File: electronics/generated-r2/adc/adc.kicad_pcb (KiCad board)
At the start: 2 copper layers, 80 x 50 mm, 22 parts, among them J1 SPI_POWER, J2 8X_HALL_3V3_GND_SIGNAL, U1 MCP3208-BI/SL, U2 SN74LVC1G125DBVR_IOFF

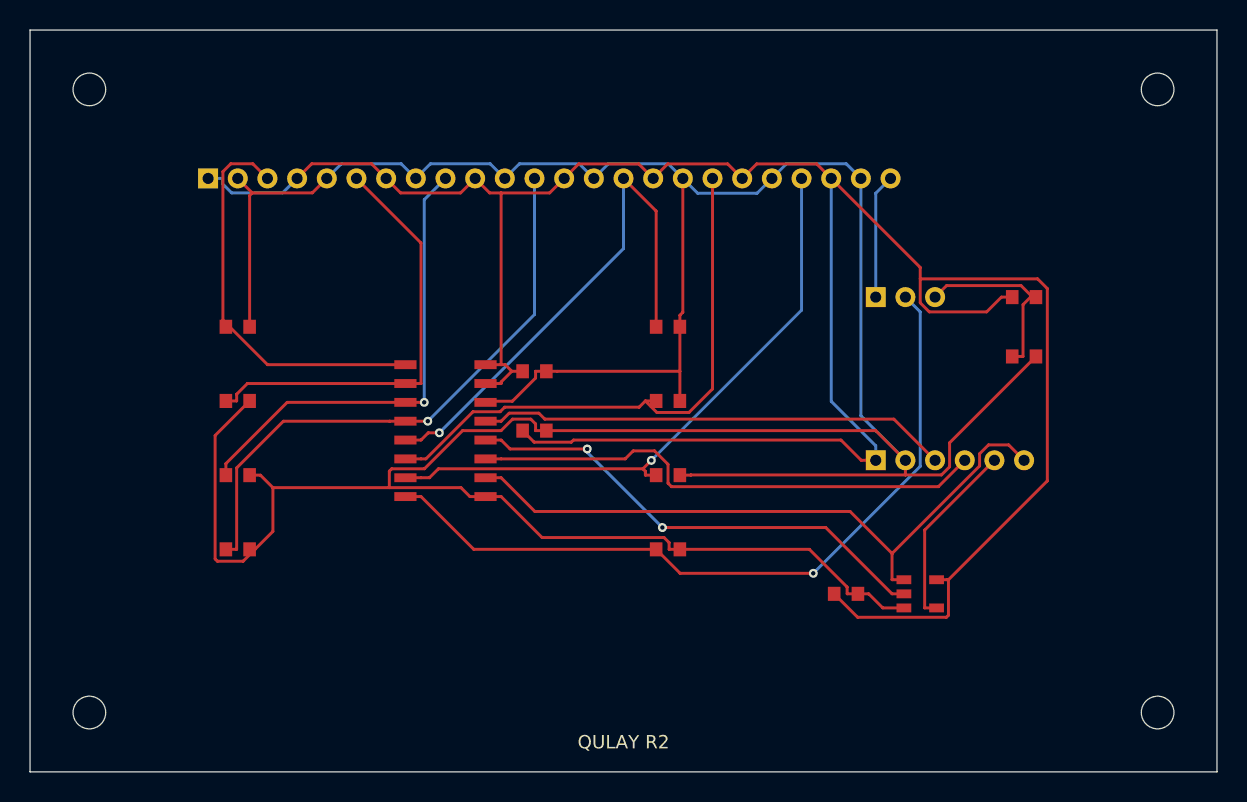
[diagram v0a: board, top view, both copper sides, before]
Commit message: build(r2): publish final routed electronics and checks [skip ci]
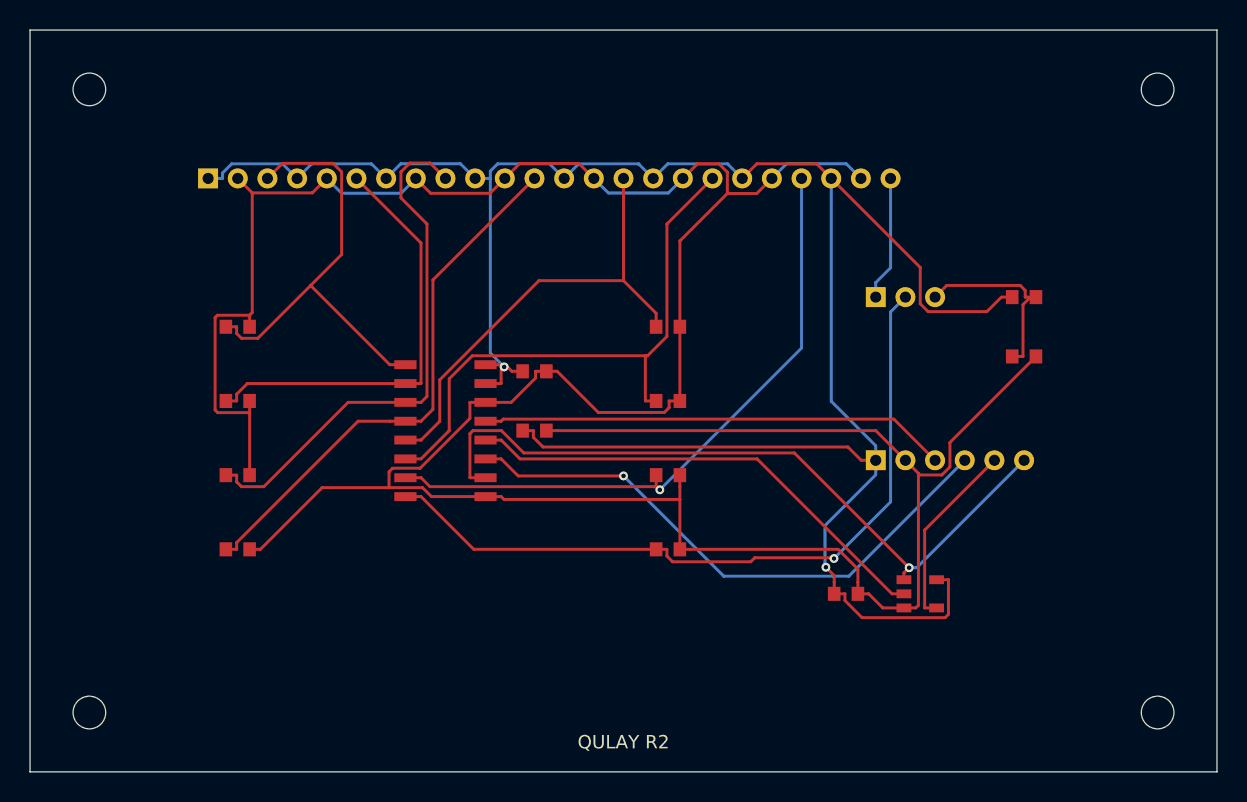
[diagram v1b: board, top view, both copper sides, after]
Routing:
- net GND: track 242.4 -> 218.1 mm
- net SENS_3V3: track 169.9 -> 151.6 mm, vias 0 -> 2
- net A2: track 31.5 -> 36.2 mm, vias 1 -> 0
- net ADC_CS: track 44.9 -> 49.2 mm, vias 0 -> 1
- net A4: track 35.7 -> 31.7 mm, vias 1 -> 0
- net ADC_MOSI: track 35.0 -> 38.8 mm, vias 0 -> 1
- net A3: track 39.7 -> 36.5 mm, vias 1 -> 0
- net A0: track 27.4 -> 30.6 mm
- net A6: track 41.5 -> 43.2 mm
- net A7: track 51.7 -> 50.7 mm
- net A5: track 38.2 -> 38.8 mm
- net ADC_OUT_RAW: track 32.6 -> 32.5 mm, vias 2 -> 0

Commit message: build(r2): publish four routed boards and checks [skip ci]
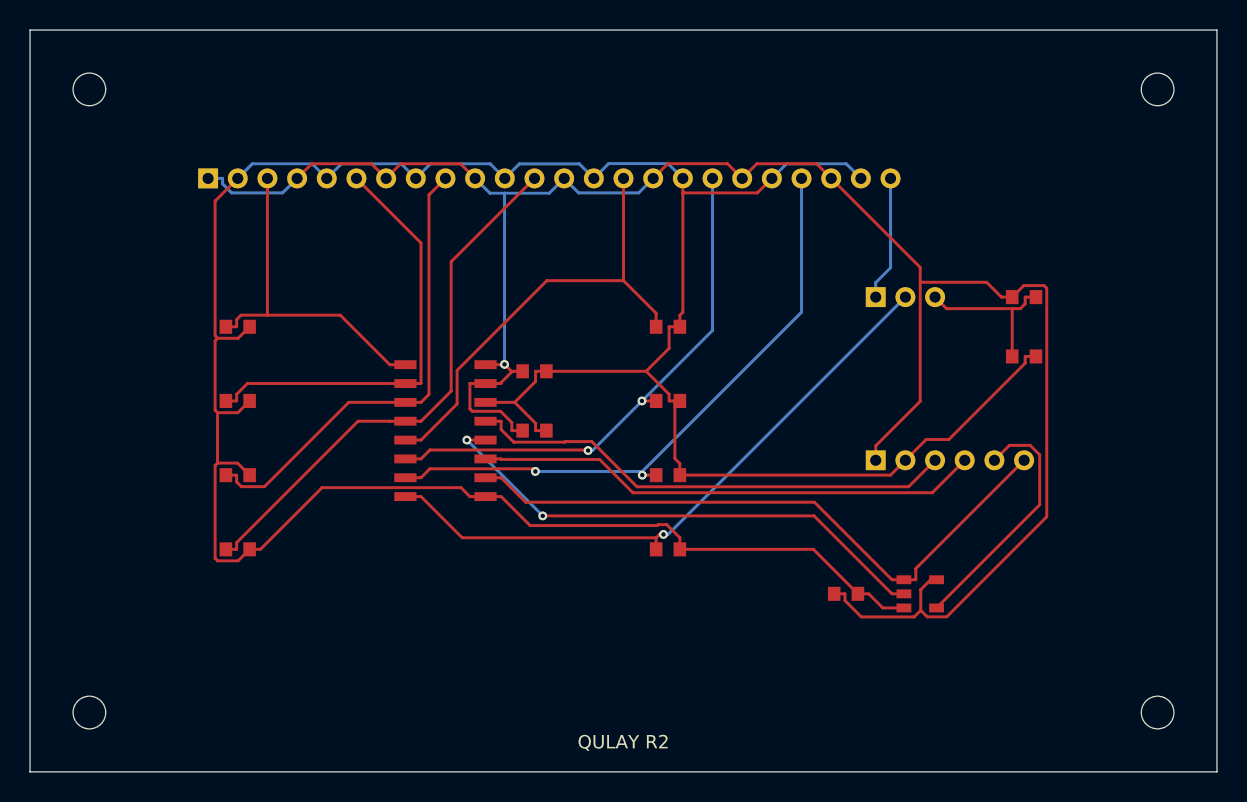
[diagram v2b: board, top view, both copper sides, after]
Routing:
- net GND: track 218.1 -> 199.5 mm
- net SENS_3V3: track 151.6 -> 140.2 mm, vias 2 -> 1
- net A7: track 50.7 -> 42.3 mm
- net A0: track 30.6 -> 23.3 mm
- net ADC_CS: track 49.2 -> 42.9 mm, vias 1 -> 0
- net ADC_MOSI: track 38.8 -> 34.2 mm, vias 1 -> 0
- net A2: track 36.2 -> 31.9 mm
- net ADC_MISO: track 12.7 -> 16.9 mm
- net A5: track 38.8 -> 35.5 mm, vias 0 -> 2
- net ADC_OUT_RAW: track 32.5 -> 35.0 mm, vias 0 -> 2
- net MID: track 12.7 -> 10.9 mm
- net ADC_SCK: track 31.5 -> 33.2 mm
- net A6: track 43.2 -> 41.7 mm, vias 1 -> 2
